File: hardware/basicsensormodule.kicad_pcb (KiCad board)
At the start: 2 copper layers, 52.1 x 121 mm, 38 parts, among them J1 Conn_01x04, J401 USART, J501 Raspberry_Pi_2_3, J601 RJ45, J602 RJ45, U201 MCP2551-I/SN, U202 MCP2515-xSO, U501 LM7805, Y201 16MHz

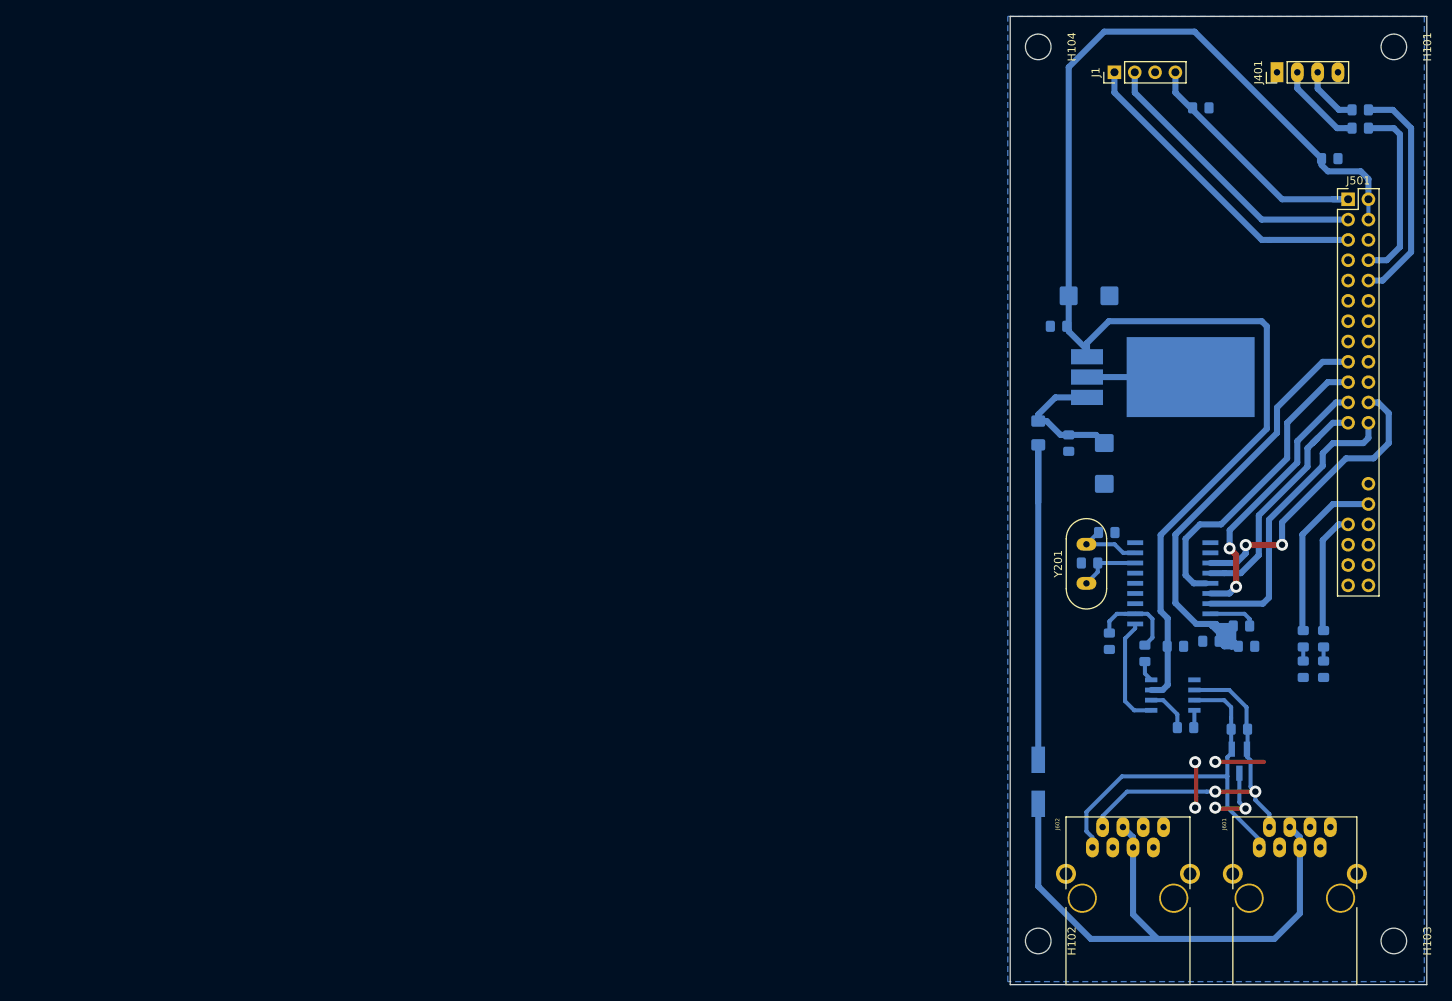
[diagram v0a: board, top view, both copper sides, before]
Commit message: Project cleaned
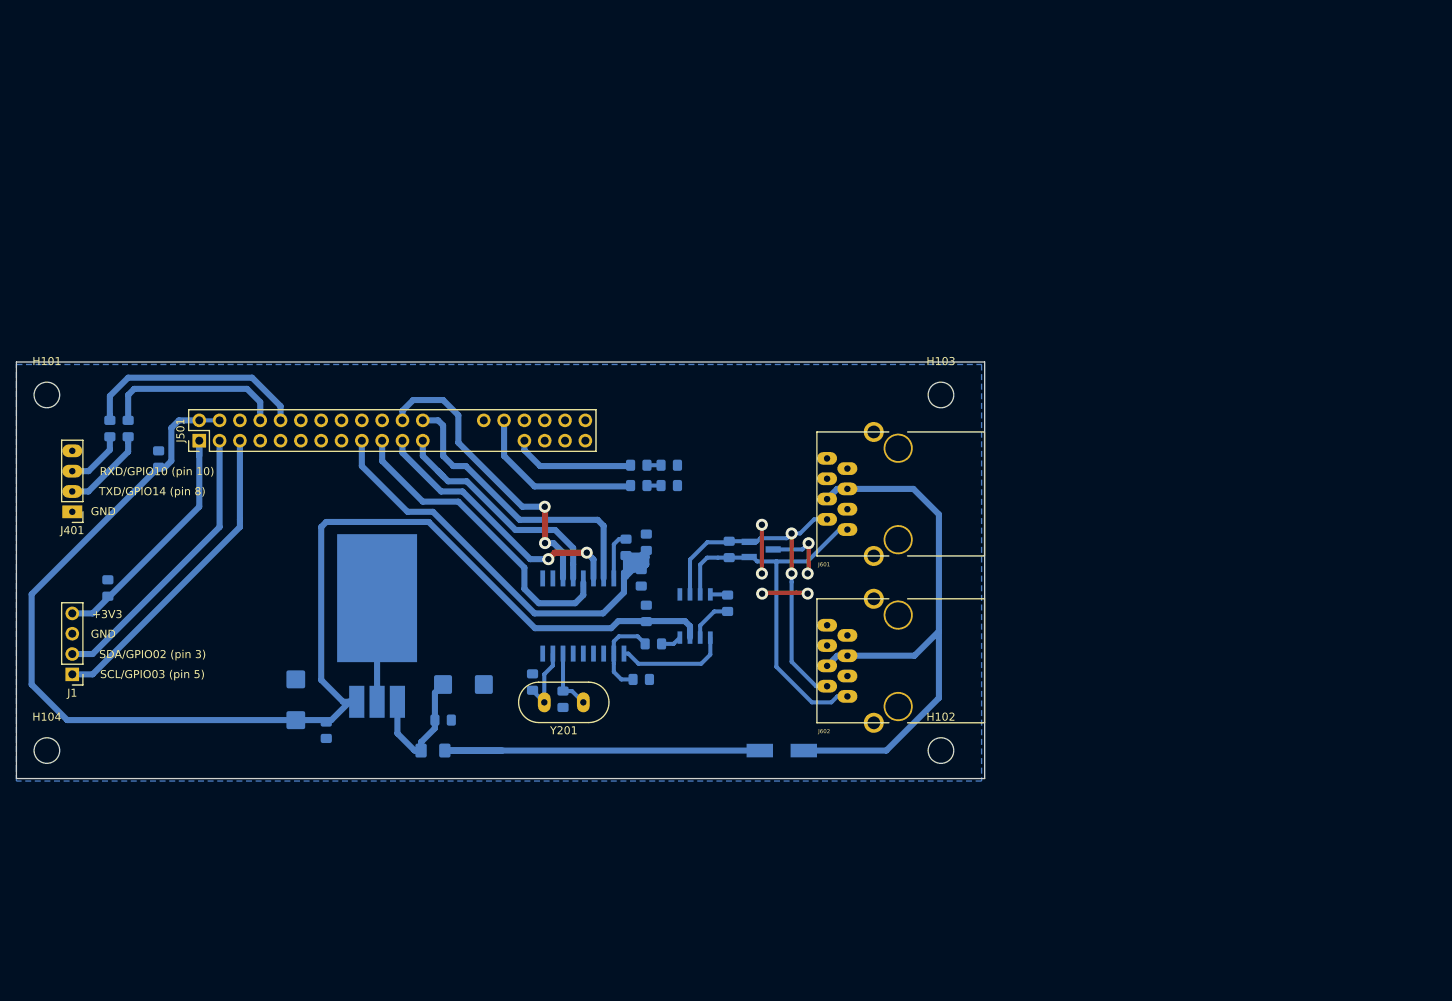
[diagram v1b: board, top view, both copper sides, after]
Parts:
- J1: value Conn_01x04 -> I2C
- moved H101 173.9 mm to (97.1, 79.1), turned to 0 degrees
- moved R402 161.3 mm to (104.9, 83.3), turned to 270 degrees
- moved J401 160.3 mm to (100.2, 93.7), turned to 180 degrees
- moved R403 158.5 mm to (107.2, 83.3), turned to 270 degrees
- moved H104 152.0 mm to (97.1, 123.5), turned to 0 degrees
- moved C401 151.1 mm to (111.0, 87.1), turned to 90 degrees
- moved J1 150.4 mm to (100.2, 114.0), turned to 180 degrees
- moved C102 149.2 mm to (104.7, 103.2), turned to 90 degrees
- moved J501 146.7 mm to (116.1, 84.8), turned to 90 degrees
- moved C504 111.3 mm to (128.2, 117.2), turned to 90 degrees
- moved C503 104.5 mm to (132.0, 121.0), turned to 270 degrees
- moved U501 94.9 mm to (140.9, 116.2), turned to 180 degrees
- moved H103 88.7 mm to (208.8, 79.1), turned to 0 degrees
- moved R404 88.3 mm to (171.0, 87.9), turned to 0 degrees
- moved D402 85.7 mm to (174.9, 87.9), turned to 180 degrees
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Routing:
- net (no net): vias 0 -> 1
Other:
- board size 52.1 x 121 mm -> 121 x 52.1 mm
- board text added: "+3V3"
- board text added: "GND"
- board text added: "RXD/GPIO10 (pin 10)"
- board text added: "SCL/GPIO03 (pin 5)"
- board text added: "SDA/GPIO02 (pin 3)"
- board text added: "TXD/GPIO14 (pin 8)"
